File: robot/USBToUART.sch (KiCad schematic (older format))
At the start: 11 parts, among them Q1 BC849, Q2 BC849, U3 CH340G, Y1 Crystal_GND24

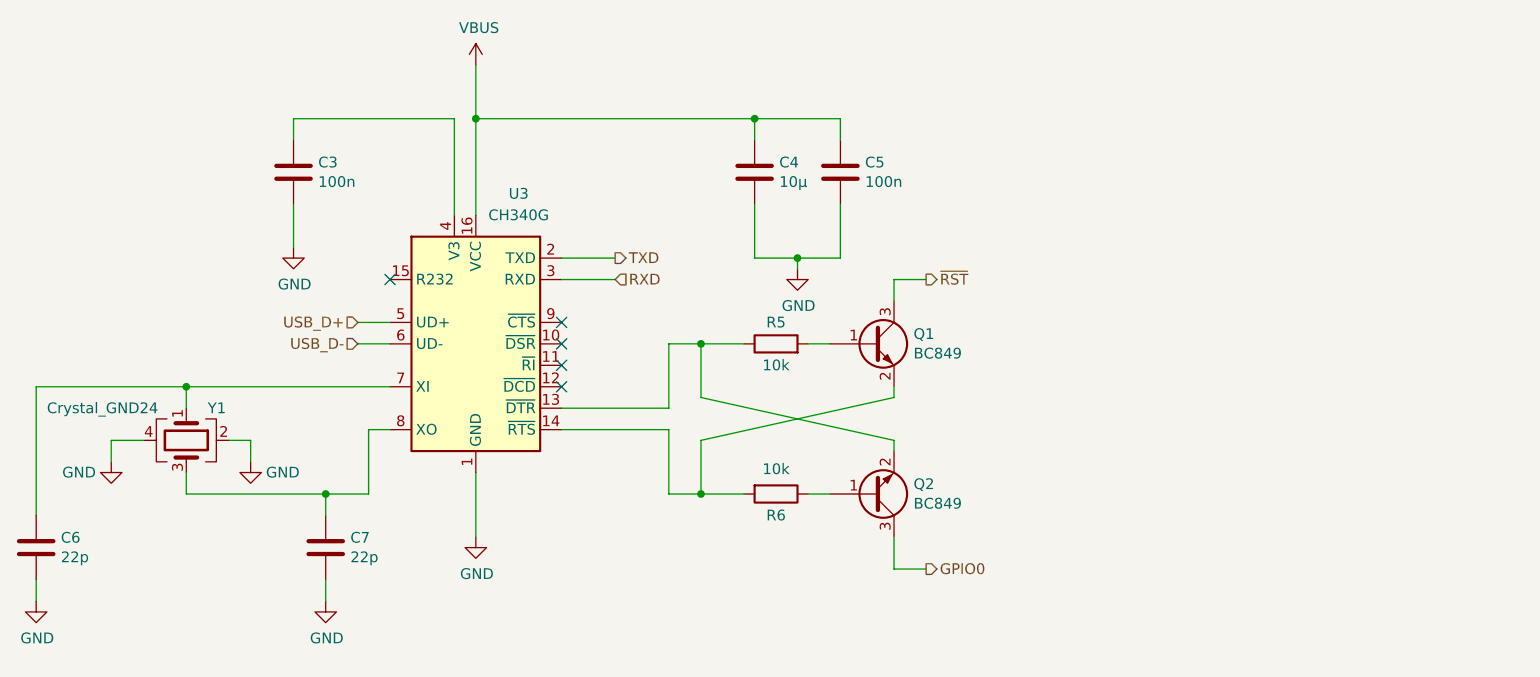
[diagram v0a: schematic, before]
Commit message: Testpoints, switch, small changes
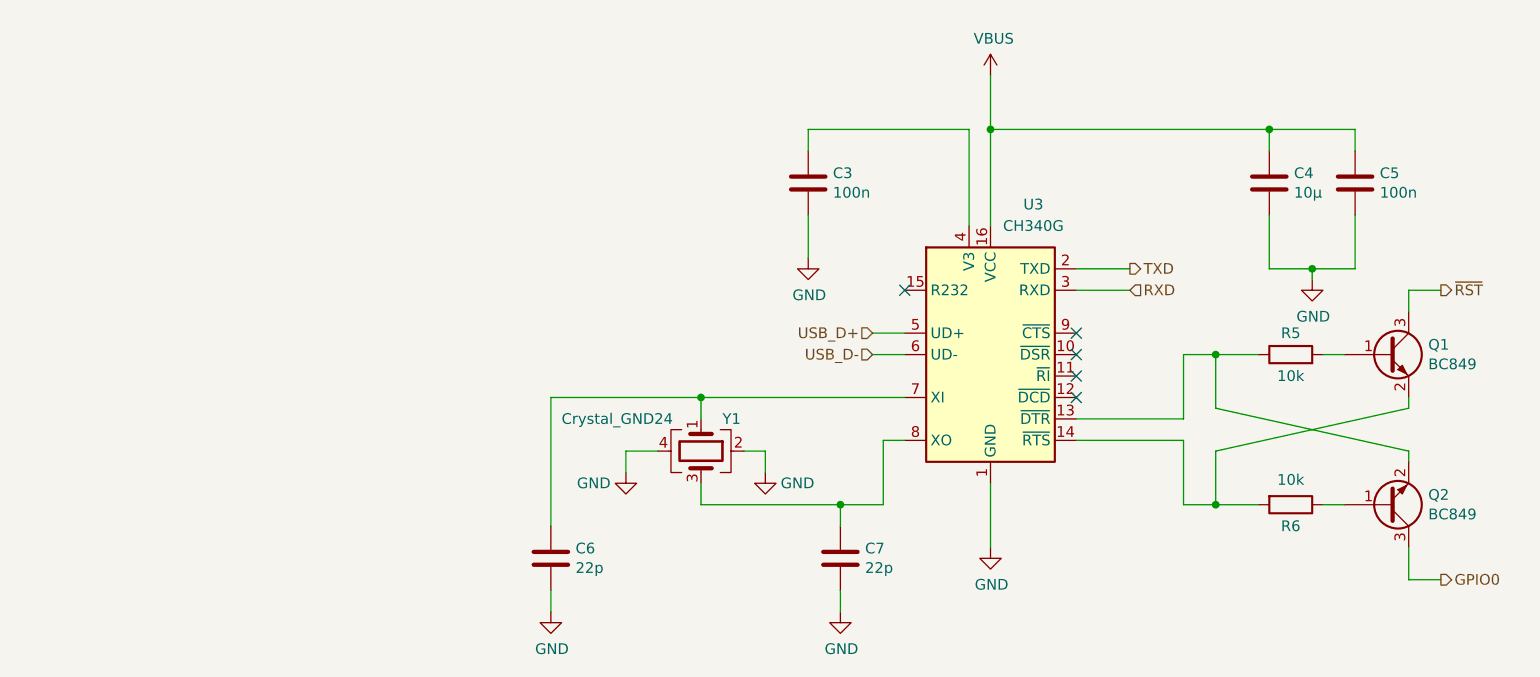
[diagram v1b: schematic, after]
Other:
- moved on the sheet: C3, C4, C5, C6, C7, Q1, Q2, R5, R6, U3, Y1
